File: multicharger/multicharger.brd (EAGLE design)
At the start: 26 x 52 mm, 26 parts, among them J2 USB-MICROA-AMPHENOL-10118192-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, J3 HEADER-8POS-, P1 TEST-POINT, P2 TEST-POINT, P3 TEST-POINT, P4 TEST-POINT, P5 TEST-POINT, P6 TEST-POINT, U1 MCP73831T-2ACI/OT, U2 MCP73831T-2ACI/OT, U3 MCP73831T-2ACI/OT, U4 MCP73831T-2ACI/OT

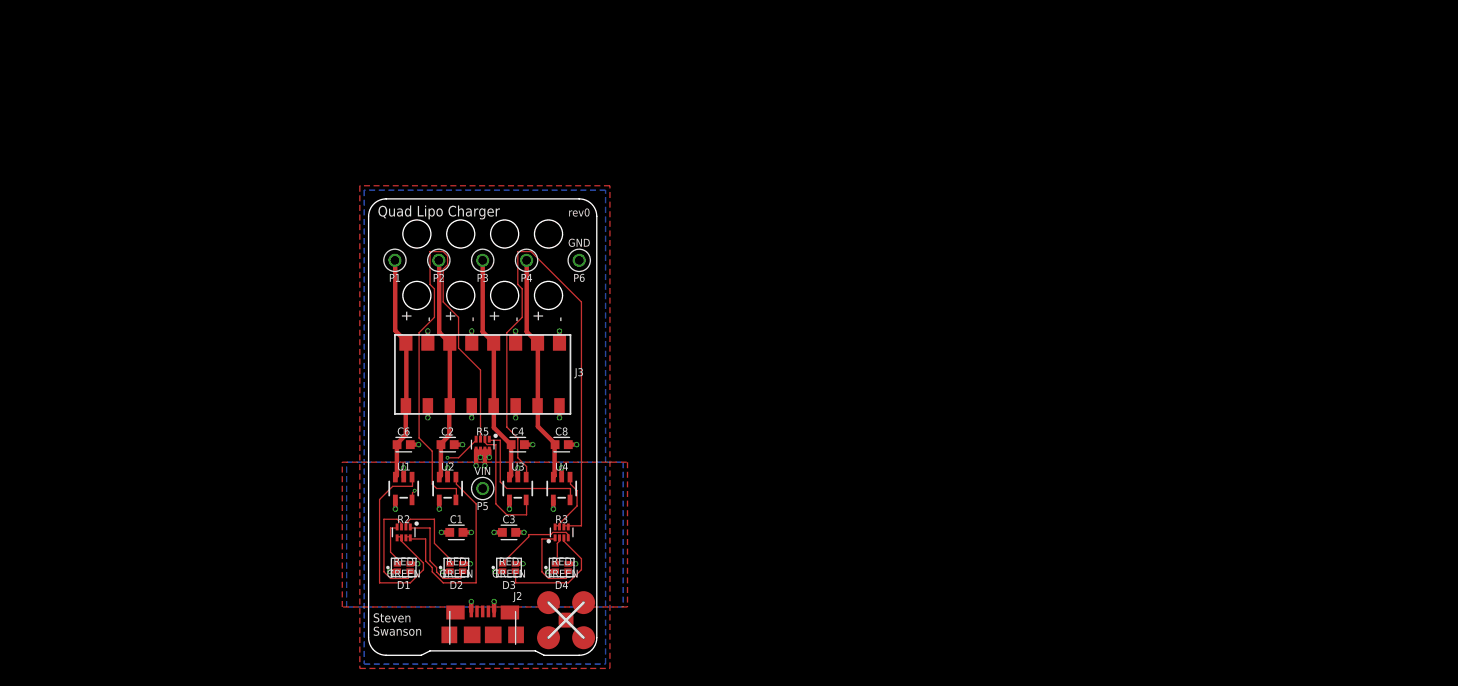
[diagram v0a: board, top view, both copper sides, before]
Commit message: Bigger resistors on leds
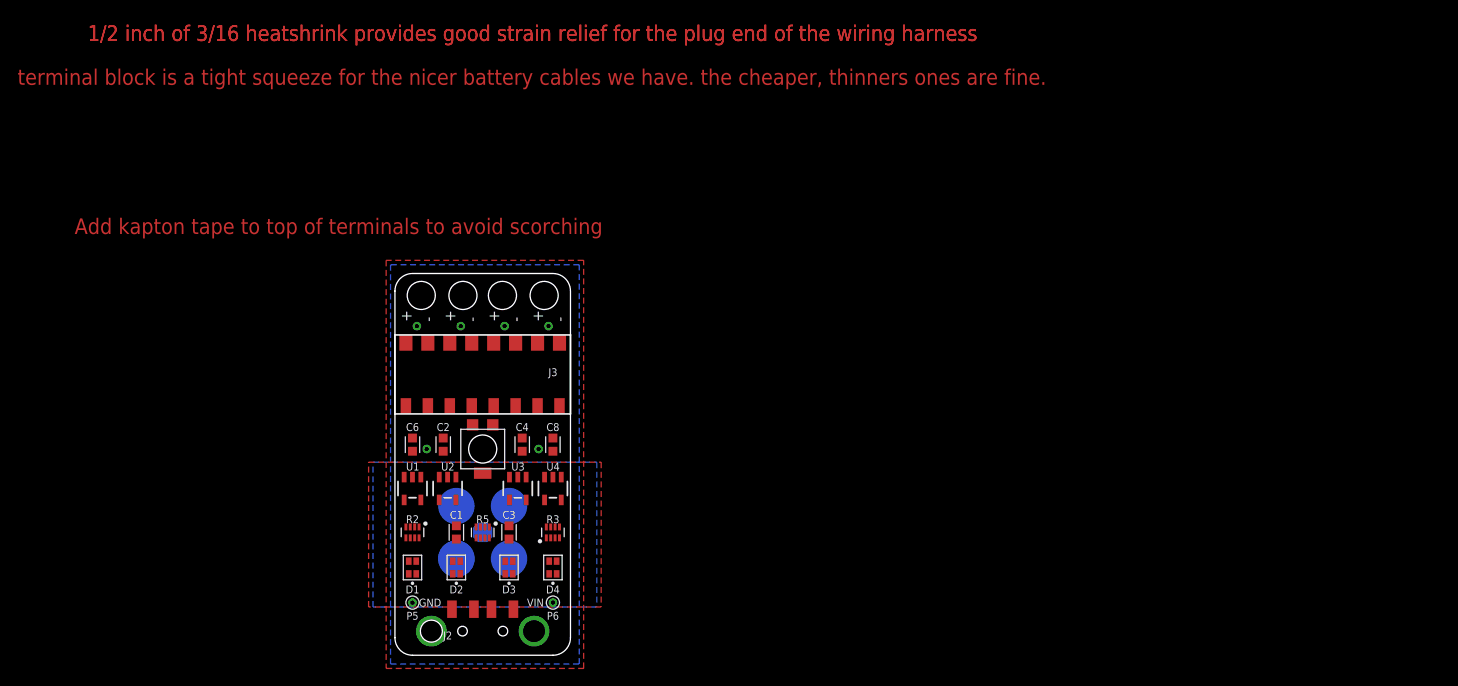
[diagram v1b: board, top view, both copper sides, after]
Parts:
- removed U$1: (no value), quadparts_prebuilt:QUADCLASS_LOGO_SMALL
- added P7: 10K, RemoteParts:BOT-ADJUST-POT-3314R-1-103E
- added P8, P9: TEST-POINT-1MM, RemoteParts:TEST-POINT-1MM-VIA
- added U$2: (no value), quadparts_prebuilt:QUADCLASS_LOGO
- J2: value USB-MICROA-AMPHENOL-10118192-0001LF -> USB-A-SMD-KEYSTONE-931; device RemoteParts:USB-MICROA-10118192-0001LF -> RemoteParts:USB-A-KEYSTONE-931
- P1, P2, P3, P4, P5, P6: value TEST-POINT -> TEST-POINT-1MM; device RemoteParts:TEST-POINT-KEYSTONE-5000 -> RemoteParts:TEST-POINT-1MM-VIA
- R2, R3: value 510 -> 750
- moved P6 39.1 mm to (8.00, -16.0)
- moved P5 15.3 mm to (-8.00, -16.0)
- moved R5 10.0 mm to (0.00, -8.00)
- moved P1 7.91 mm to (-7.50, 15.5), flipped to the bottom
- moved P2 7.91 mm to (-2.50, 15.5), flipped to the bottom
- moved P3 7.91 mm to (2.50, 15.5), flipped to the bottom
- moved P4 7.91 mm to (7.50, 15.5), flipped to the bottom
- moved C6 1.00 mm to (-8.00, 2.00), turned to 90 degrees
- moved C8 1.00 mm to (8.00, 2.00), turned to 90 degrees
- moved D1 1.00 mm to (-8.00, -12.0), turned to 270 degrees
- moved D4 1.00 mm to (8.00, -12.0), turned to 270 degrees
- moved J2 1.00 mm to (0.00, -18.0), turned to 180 degrees
- moved R2 1.00 mm to (-8.00, -8.00)
- moved R3 1.00 mm to (8.00, -8.00)
- moved U1 1.00 mm to (-8.00, -3.00)
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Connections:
- new net N$17: P7.1, P8.T
- new net N$18: P7.3, P9.T
- net GND: now also J2.G1, J2.G2; no longer J2.10, J2.11, J2.5, J2.6, J2.7, J2.8, J2.9
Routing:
- net N$7: track 65.0 -> 0.00 mm
- net N$4: track 57.4 -> 0.00 mm
- net GND: track 30.5 -> 0.00 mm, vias 27 -> 0
- net BPOS3: track 26.1 -> 0.00 mm
- net BPOS4: track 26.1 -> 0.00 mm
- net N$11: track 26.0 -> 0.00 mm
- net BPOS1: track 25.7 -> 0.00 mm
- net BPOS2: track 25.7 -> 0.00 mm
- net N$3: track 25.2 -> 0.00 mm
- net N$14: track 15.8 -> 0.00 mm
- net N$8: track 14.2 -> 0.00 mm
- net N$9: track 13.9 -> 0.00 mm
- net N$1: track 12.6 -> 0.00 mm
- net N$5: track 11.7 -> 0.00 mm
- net VIN: track 10.7 -> 0.00 mm, vias 11 -> 0
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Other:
- board size 26 x 52 mm -> 20 x 43.5 mm
- board text added: "1/2 inch of 3/16 heatshrink provides good strain relief for the plug end of the wiring harness"
- board text added: "1kΩ: 250mA"
- board text added: "250Ω: 1000mA"
- board text added: "500Ω: 500mA"
- board text added: "Add kapton tape to top of terminals to avoid scorching"
- board text added: "Set Charging Current"
- board text added: "rev1"
- board text added: "terminal block is a tight squeeze for the nicer battery cables we have. the cheaper, thinners ones are fine."
- board text removed: "rev0"
